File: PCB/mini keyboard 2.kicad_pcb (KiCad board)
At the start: 2 copper layers, 98.5 x 40.6 mm, 13 parts, among them SW1 SW_Push, SW2 SW_Push, SW3 SW_Push, SW4 SW_Push, SW5 SW_Push, SW6 SW_Push, SW7 SW_Push, SW8 SW_Push, SW9 RotaryEncoder_Switch, U1 XIAO-RP2040-DIP

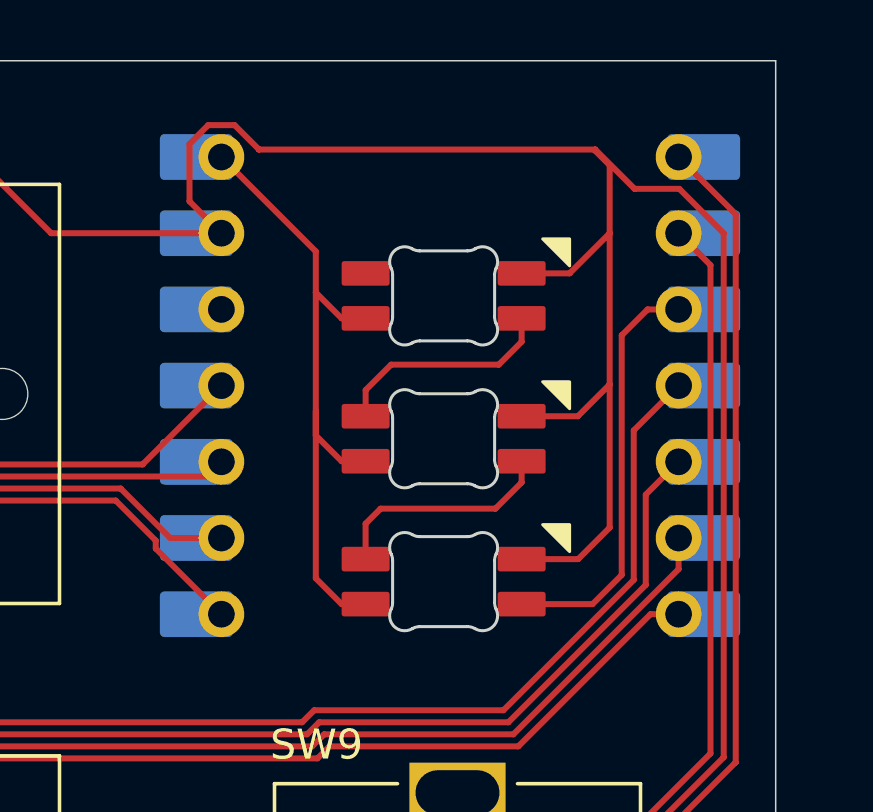
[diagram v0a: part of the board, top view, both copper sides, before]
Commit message: Update files
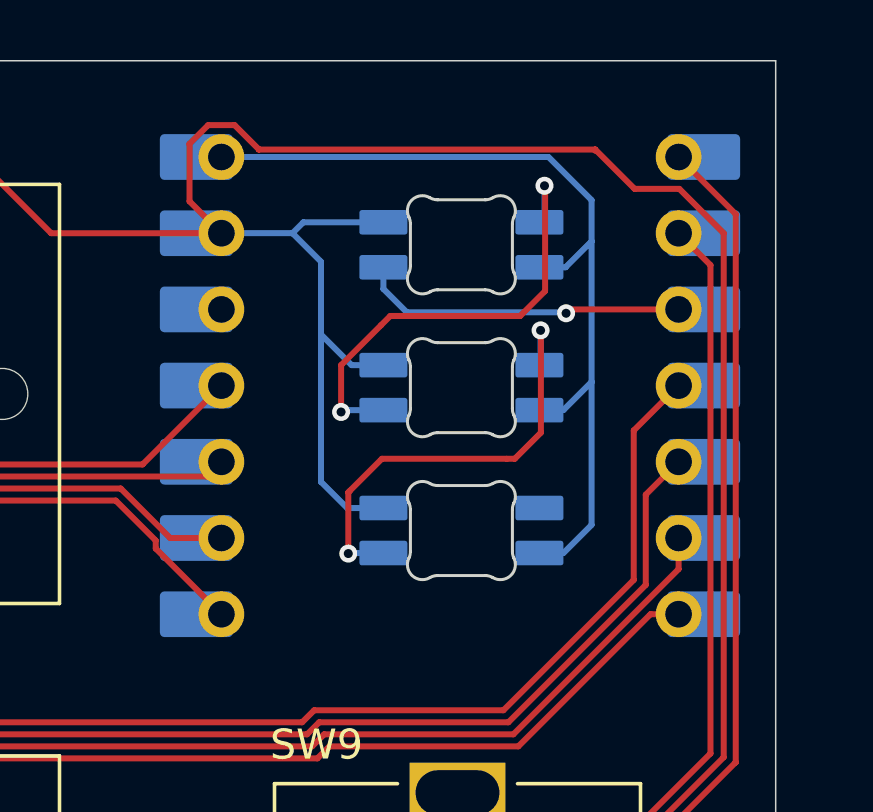
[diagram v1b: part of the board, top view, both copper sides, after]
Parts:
- D1, D2, D3: moved to F.Cu
- moved D1 11.2 mm to (128.8, 25.1), turned to 0 degrees
- moved D3 7.84 mm to (128.8, 34.7), turned to 0 degrees
- moved D2 1.80 mm to (128.8, 29.9), turned to 0 degrees
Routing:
- net Net-(D1-DOUT): track 7.66 -> 15.6 mm, vias 0 -> 2
- net +5V: track 22.2 -> 30.1 mm
- net Net-(D2-DOUT): track 7.52 -> 15.1 mm, vias 0 -> 2
- net GND: track 261.9 -> 258.1 mm
- net Net-(D1-DIN): track 14.0 -> 11.0 mm, vias 0 -> 1
